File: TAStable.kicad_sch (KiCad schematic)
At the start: 18 parts, among them J1 IN/OUT, J2 ICSP, U1 74HCT1G04, U2 CS2300-CP, U3 74LVC1G14, U4 PIC16LF15313, U6 AZ1117-3.3

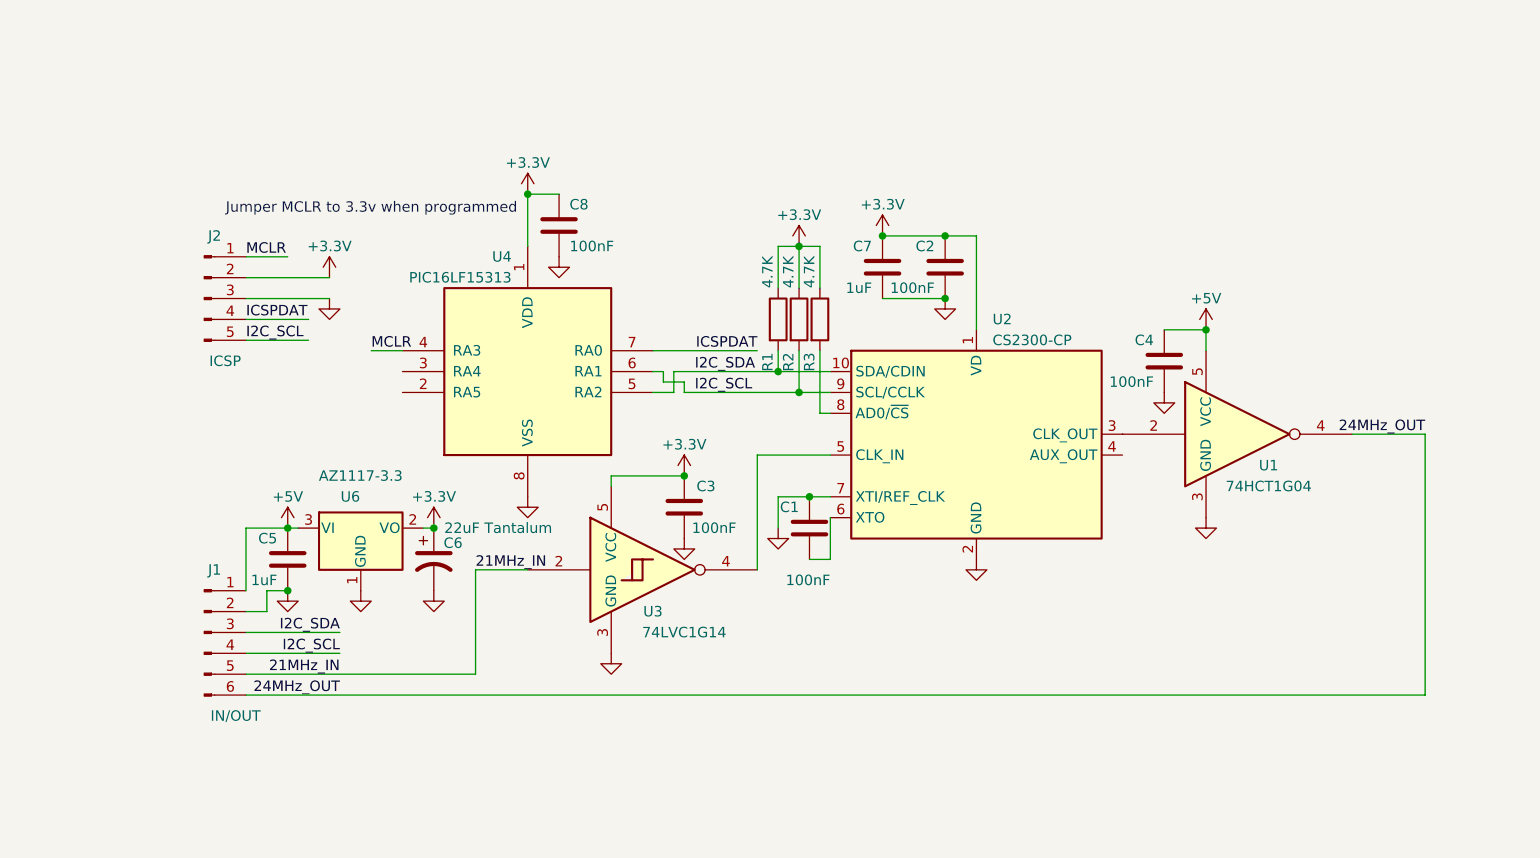
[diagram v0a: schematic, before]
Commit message: v2
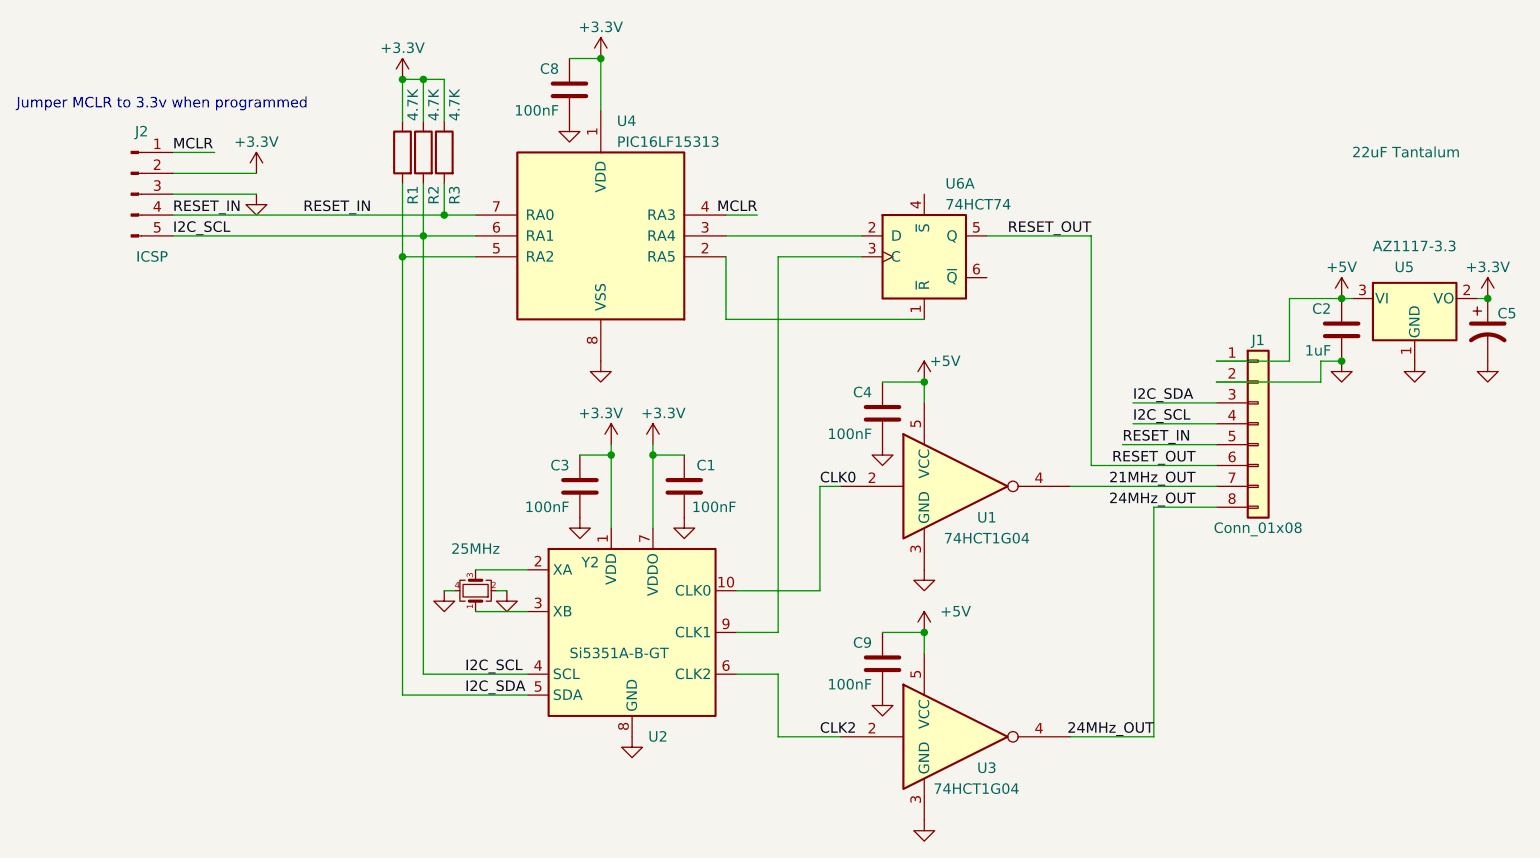
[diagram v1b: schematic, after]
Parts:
- removed C5, C7: 1uF, Capacitor_SMD:C_0603_1608Metric, symbol Device:C
- removed C6: 22uF Tantalum, Capacitor_SMD:C_1206_3216Metric, symbol Device:C_Polarized_US
- removed J1: IN/OUT, Connector_PinHeader_2.54mm:PinHeader_1x06_P2.54mm_Horizontal, symbol Connector:Conn_01x06_Pin
- removed U2: CS2300-CP, Package_SO:MSOP-10_3x3mm_P0.5mm, symbol Timer_PLL:CS2000-CP
- removed U3: 74LVC1G14, Package_TO_SOT_SMD:SOT-353_SC-70-5, symbol 74xGxx:74LVC1G14
- removed U6: AZ1117-3.3, Package_TO_SOT_SMD:SOT-89-3, symbol Regulator_Linear:AZ1117-3.3
- added C5: 22uF Tantalum, Capacitor_SMD:C_1206_3216Metric, symbol Device:C_Polarized_US
- added C9: 100nF, Capacitor_SMD:C_0603_1608Metric, symbol Device:C
- added J1: Conn_01x08, symbol Connector_Generic:Conn_01x08
- added U2: Si5351A-B-GT, Package_SO:MSOP-10_3x3mm_P0.5mm, symbol Oscillator:Si5351A-B-GT
- added U3: 74HCT1G04, Package_TO_SOT_SMD:SOT-353_SC-70-5, symbol 74xGxx:74AHCT1G04
- added U5: AZ1117-3.3, Package_TO_SOT_SMD:SOT-89-3, symbol Regulator_Linear:AZ1117-3.3
- added U6: 74HCT74, symbol 74xx:74HC74
- added Y2: 25MHz, symbol Device:Crystal_GND24_Small
- C2: value 100nF -> 1uF
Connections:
- net ICSPDAT is gone; now on net RESET_IN: J2.4 (Pin_4), U4.7 (RA0)
- net +3.3V: now also C1.1, C5.1, U2.1 (VDD), U2.7 (VDDO), U5.2 (VO); no longer C2.1
- net +5V: now also C2.1, C9.1, J1.1 (Pin_1), U3.5 (VCC), U5.3 (VI)
- net 24MHz_OUT: now also J1.8 (Pin_8), U3.4; no longer U1.4
- net GND: now also C1.2, C5.2, C9.2, J1.2 (Pin_2), U2.8 (GND), U3.3 (GND), U5.1 (GND), Y2.2, Y2.4; no longer C1.1
- net I2C_SCL: now also J1.4 (Pin_4), U2.4 (SCL)
- net I2C_SDA: now also J1.3 (Pin_3), U2.5 (SDA)
- net CLK0: now reaches U1.2
- net CLK0: now also U2.10 (CLK0)
- net RESET_IN: now reaches R3.2
- net RESET_IN: now also J1.5 (Pin_5)
- net at U4.2 (RA5): now also U6.1 (~{R})
- net at U4.3 (RA4): now also U6.2 (D)
- new net: U2.2 (XA), Y2.3
- new net: U2.3 (XB), Y2.1
- new net: U2.9 (CLK1), U6.3 (C)
- new net 21MHz_OUT: J1.7 (Pin_7), U1.4
- new net CLK2: U2.6 (CLK2), U3.2
- new net RESET_OUT: J1.6 (Pin_6), U6.5 (Q)
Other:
- moved on the sheet: C4, C8, J2, R1, R2, U1, U4
